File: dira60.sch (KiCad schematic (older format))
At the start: 20 parts, among them J0 USB_C_Receptacle, SW0 RESET, U0 ATmega32U4-AU, X0 XTAL_GND

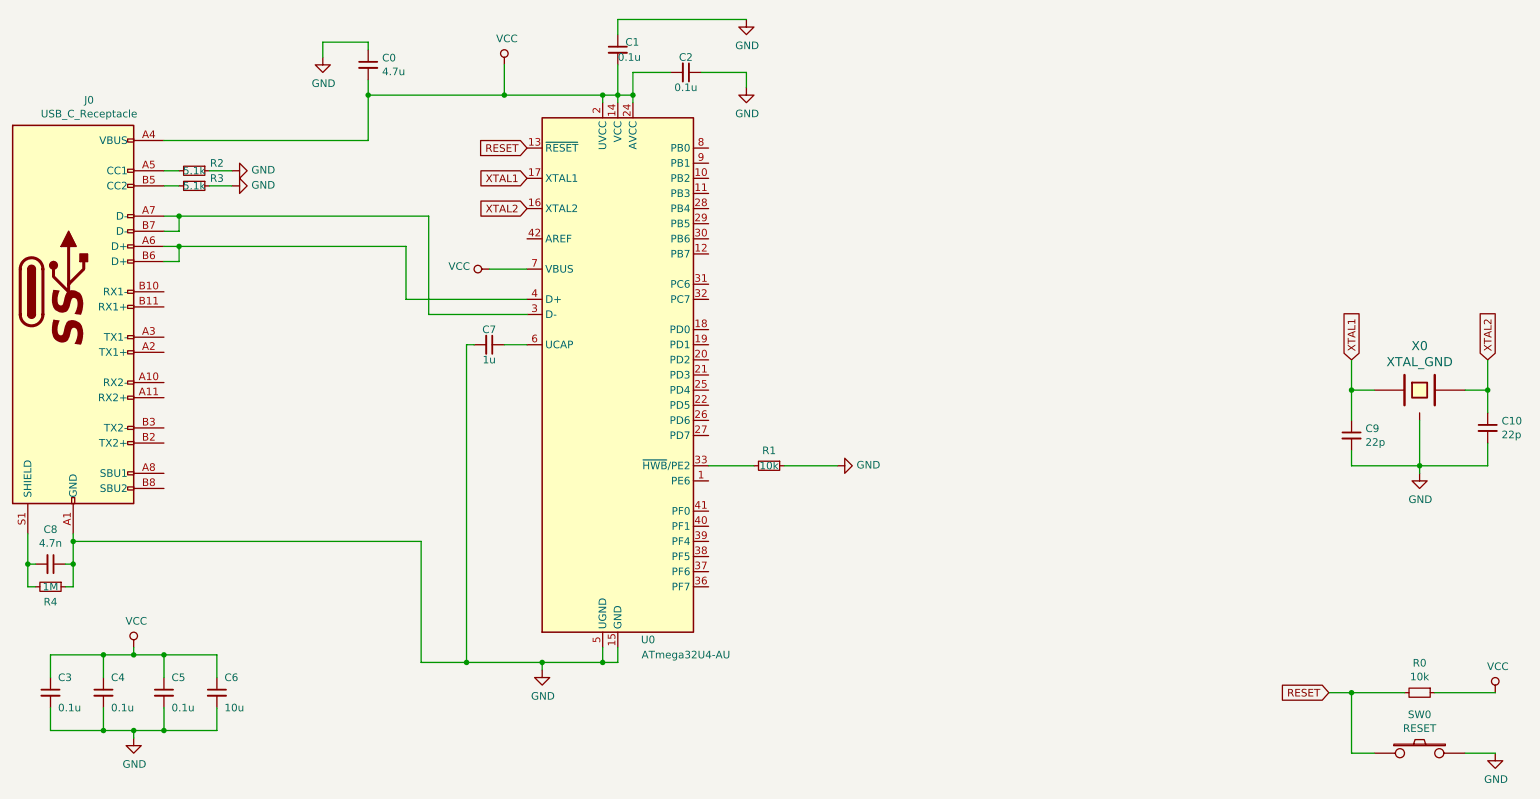
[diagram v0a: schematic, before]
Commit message: Schematic updated
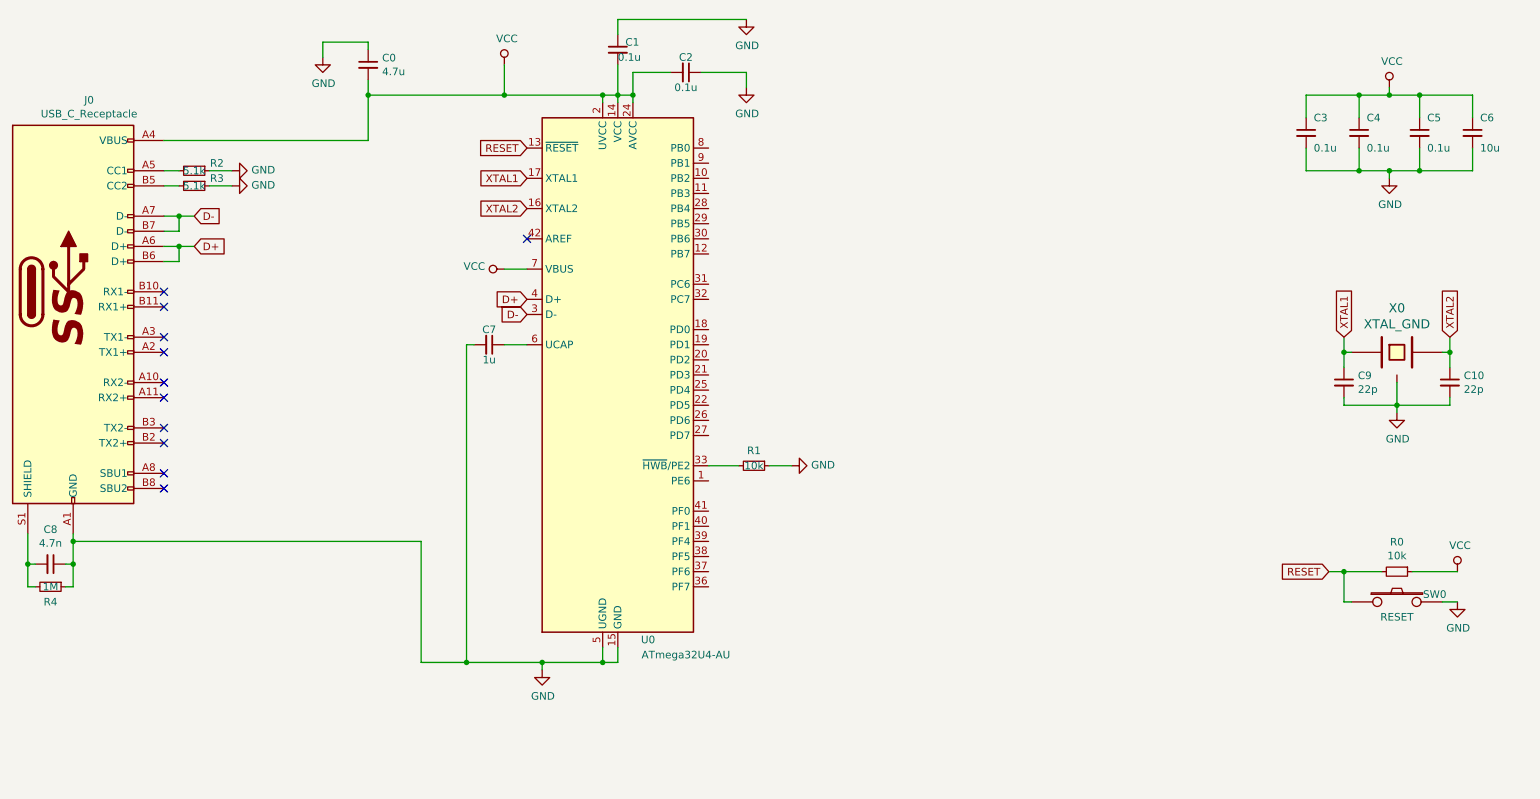
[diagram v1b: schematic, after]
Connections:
- net D-: now reaches J0.A7 (D-), J0.B7 (D-), U0.3 (D-)
- net D+: now reaches J0.A6 (D+), J0.B6 (D+), U0.4 (D+)
- no-connect marks 0 -> 11
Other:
- moved on the sheet: C10, C3, C4, C5, C6, C9, R0, R1, SW0, X0

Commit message: Updated Schematic
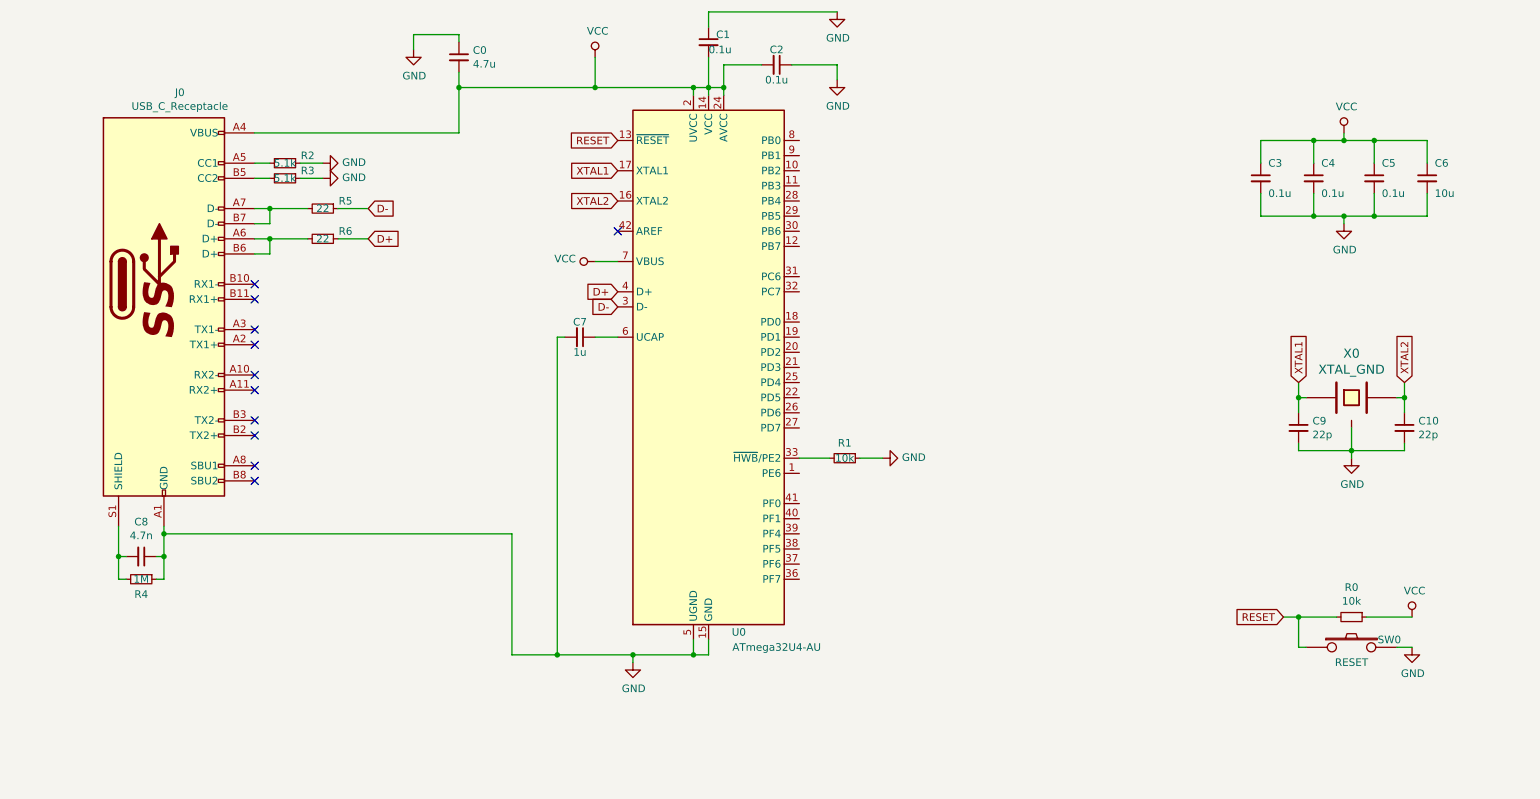
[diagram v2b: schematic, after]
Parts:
- added R5, R6: 22, symbol Device:R_Small
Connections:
- net D+: now also R6.1; no longer J0.A6 (D+), J0.B6 (D+)
- net D-: now also R5.1; no longer J0.A7 (D-), J0.B7 (D-)
- new net: J0.A6 (D+), J0.B6 (D+), R6.2
- new net: J0.A7 (D-), J0.B7 (D-), R5.2
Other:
- moved on the sheet: C0, C1, C10, C2, C3, C4, C5, C6, C7, C8, C9, J0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
